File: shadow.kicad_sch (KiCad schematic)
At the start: 10 parts, among them U1 Arduino Nano 33 IoT

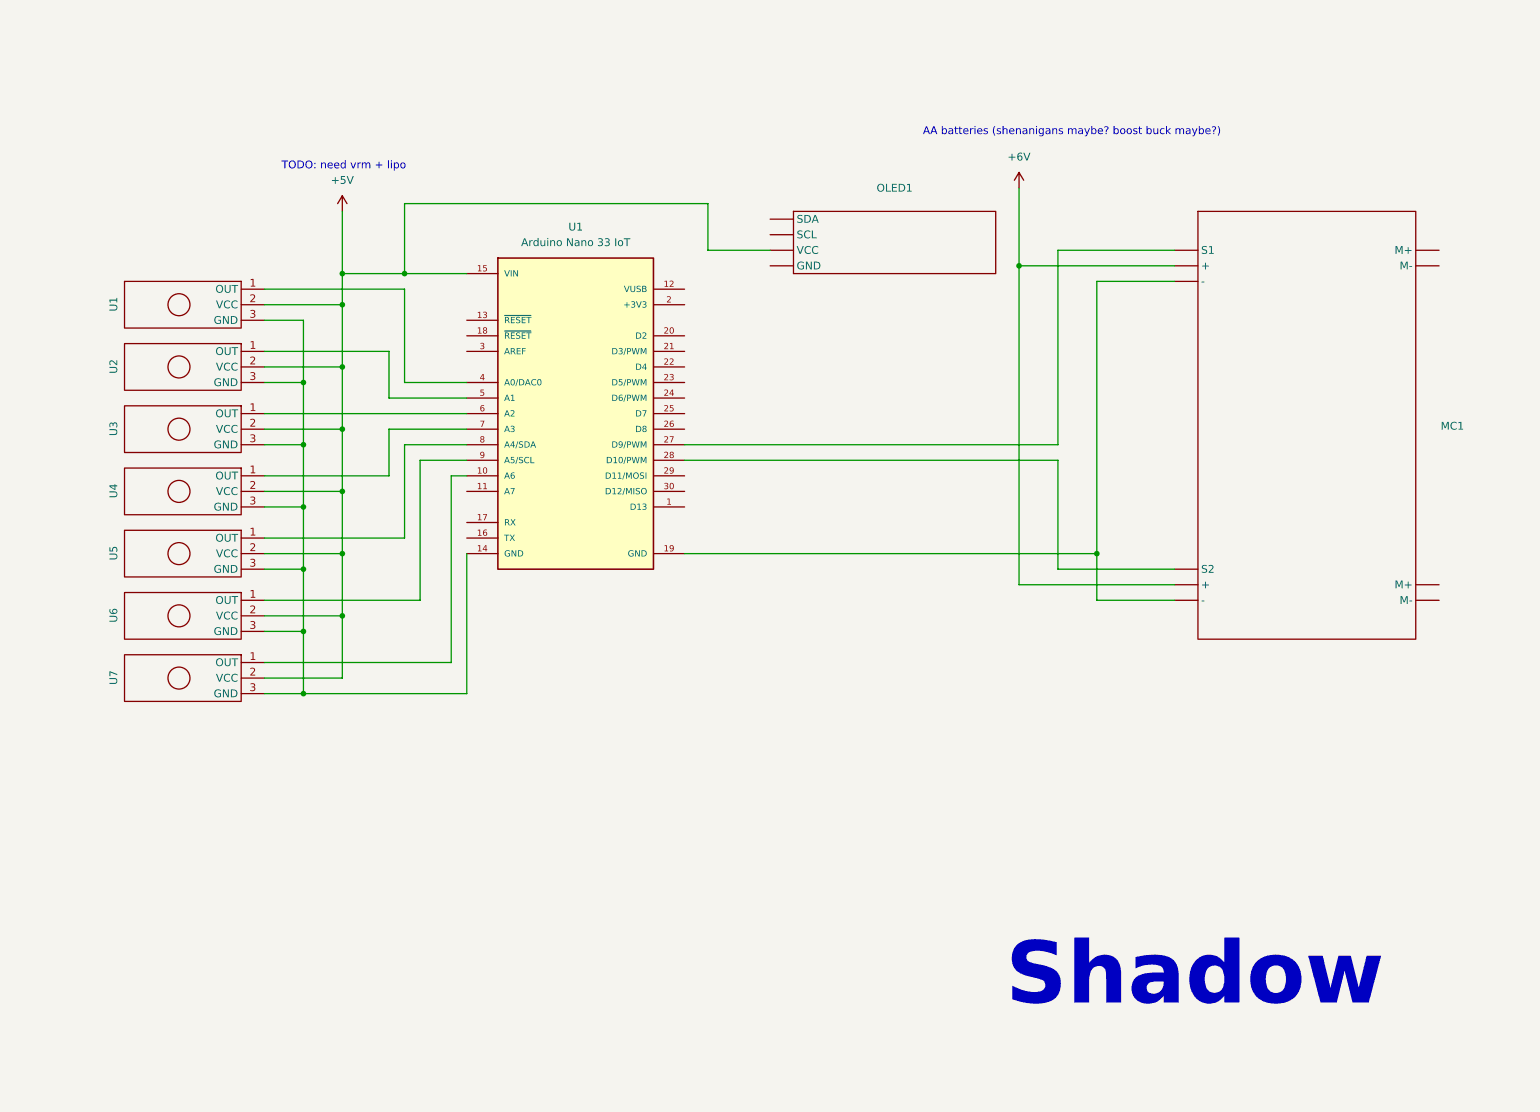
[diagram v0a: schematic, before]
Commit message: feat: finish up control circut
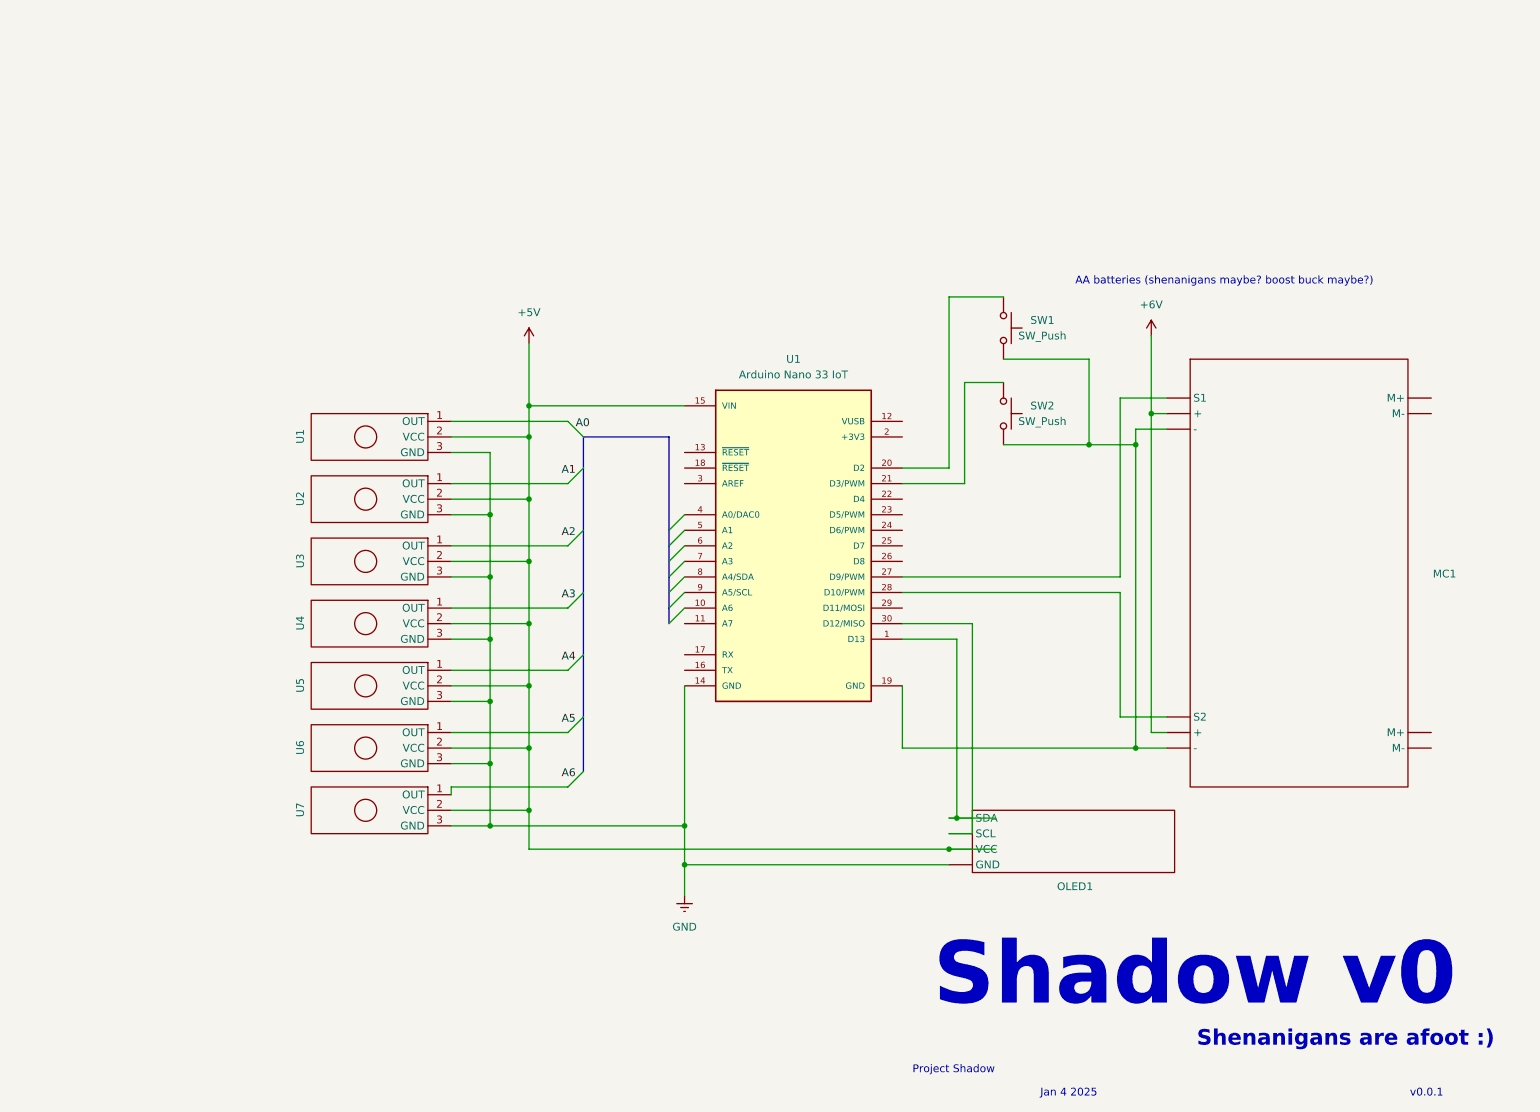
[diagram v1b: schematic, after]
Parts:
- added SW1, SW2: SW_Push, symbol Switch:SW_Push
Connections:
- net at MC1. (S2), U1.19 (GND): now also SW1.2, SW2.2
- net at U3.1 (OUT): no longer U1.6 (A2)
- net GND: now reaches U1.14 (GND), U1.3 (GND), U2.3 (GND), U3.3 (GND), U4.3 (GND), U5.3 (GND), U6.3 (GND), U7.3 (GND)
- net GND: now also OLED1. (VCC)
- net at U7.1 (OUT): no longer U1.10 (A6)
- net at U2.1 (OUT): no longer U1.5 (A1)
- net at U1.1 (D13): now also OLED1. (VCC)
- net at U1.20 (D2): now also SW1.1
- net at U1.21 (D3/PWM): now also SW2.1
- net at U1.30 (D12/MISO): now also OLED1. (VCC)
- net at U1.4 (A0/DAC0): no longer U1.1 (OUT)
- net at U1.7 (A3): no longer U4.1 (OUT)
- net at U1.8 (A4/SDA): no longer U5.1 (OUT)
- net at U1.9 (A5/SCL): no longer U6.1 (OUT)
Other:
- note added: "Jan 4 2025"
- note added: "Project Shadow"
- note added: "Shadow v0"
- note added: "Shenanigans are afoot :)"
- note added: "v0.0.1"
- note removed: "Shadow"
- note removed: "TODO: need vrm + lipo"
- moved on the sheet: MC1, OLED1, U1, U2, U3, U4, U5, U6, U7

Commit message: finish circut
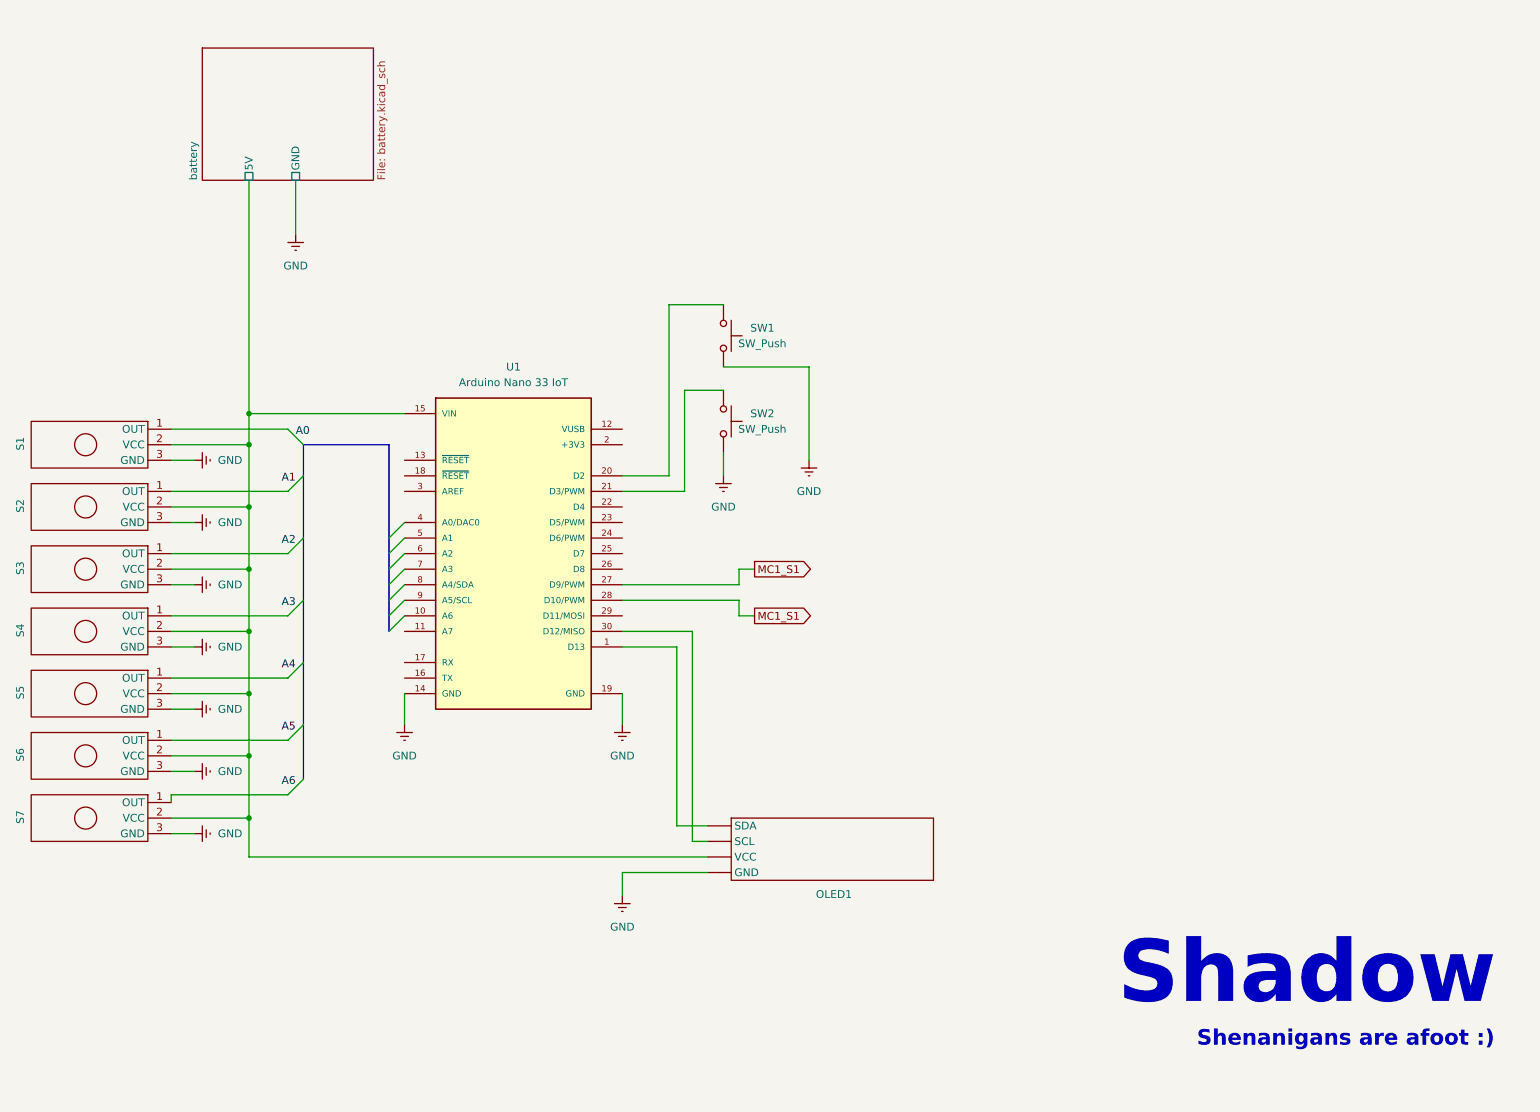
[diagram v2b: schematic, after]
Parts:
- removed MC1: ~, symbol Custom:FT-SMC-2CH
- renumbered U1 to S1, U2 to S2, U3 to S3, U4 to S4, U5 to S5, U6 to S6, U7 to S7
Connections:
- net GND: now also SW1.2, SW2.2, U1.19 (GND)
- net MC1_S1: now reaches U1.27 (D9/PWM)
- net MC1_S1: now also U1.28 (D10/PWM)
- net +5V renamed battery/5V
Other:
- added sheet battery (battery.kicad_sch)
- note added: "Shadow"
- note removed: "AA batteries (shenanigans maybe? boost buck maybe?)"
- note removed: "Jan 4 2025"
- note removed: "Project Shadow"
- note removed: "Shadow v0"
- note removed: "v0.0.1"
- company: (none) -> York Mills Collegiate Institute
- title: (none) -> Shadow
- moved on the sheet: OLED1, S1, S2, S3, S4, S5, S6, S7, SW1, SW2, U1
